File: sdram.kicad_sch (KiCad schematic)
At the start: 25 parts, among them U1 MT48LC16M16A2P, U8 T20Q144xx, X2 ECS-2520MV-250-CM

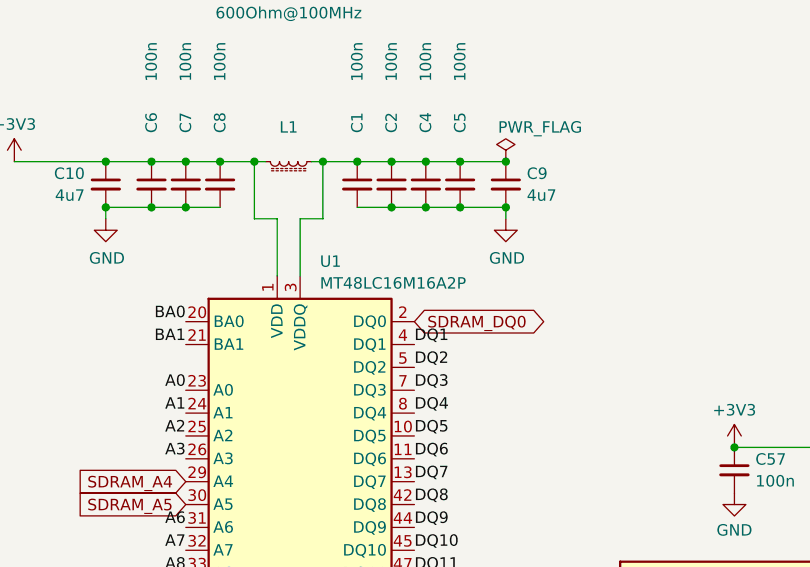
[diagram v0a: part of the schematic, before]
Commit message: part-info update
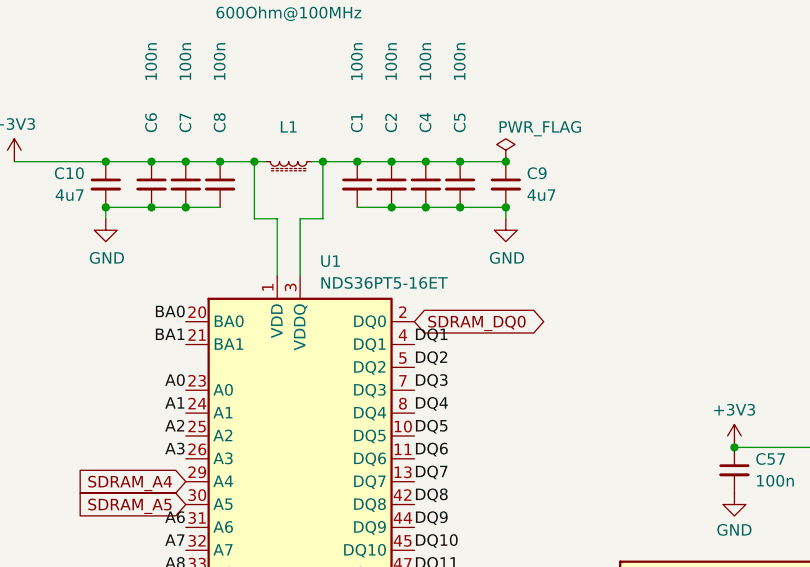
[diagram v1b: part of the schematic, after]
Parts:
- U1: value MT48LC16M16A2P -> NDS36PT5-16ET
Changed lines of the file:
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@@
       (effects (font (size 1.27 1.27)) (justify left))
     )
-    (property "Value" "MT48LC16M16A2P" (at 59.3441 54.1599 0)
+    (property "Value" "NDS36PT5-16ET" (at 59.3441 54.1599 0)
       (effects (font (size 1.27 1.27)) (justify left))
     )
@@
       (effects (font (size 1.27 1.27) italic) hide)
     )
-    (property "Datasheet" "https://www.micron.com/-/media/client/global/documents/products/data-sheet/dram/256mb_sdr.pdf" (at 57.15 95.25 0)
+    (property "Datasheet" "" (at 57.15 95.25 0)
       (effects (font (size 1.27 1.27)) hide)
     )

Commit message: Added Manufacturer + Part info for most components.
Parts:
- C1, C12, C13, C15, C2, C3, C4, C42, C5, C57, C6, C64, C7, C8: Manufacturer (none) -> Samsung; Part (none) -> CL10B104KB8NFN
- C10, C9: Manufacturer (none) -> TDK; Part (none) -> 2012X5R1C475K125AC
- L1: Manufacturer (none) -> Laird; Part (none) -> MI0603J601R-10
- U1: Manufacturer (none) -> Insignis; Part (none) -> NDS36PT5-16ET
- U8: Manufacturer (none) -> Efinix; Part (none) -> T20Q144C4
- X2: Manufacturer (none) -> ECS; Part (none) -> ECS-2520MV-250-CL-TR
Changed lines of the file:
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@@
+      (effects (font (size 1.27 1.27)) hide)
+    )
+    (property "Manufacturer" "TDK" (at 80.01 43.18 0)
+      (effects (font (size 1.27 1.27)) hide)
+    )
+    (property "Part" "2012X5R1C475K125AC" (at 80.01 43.18 0)
       (effects (font (size 1.27 1.27)) hide)
     )
@@
     )
     (property "Datasheet" "https://www.efinixinc.com/docs/trion8-ds-v4.4.pdf" (at 118.11 119.38 0)
+      (effects (font (size 1.27 1.27)) hide)
+    )
+    (property "Manufacturer" "Efinix" (at 118.11 92.71 0)
+      (effects (font (size 1.27 1.27)) hide)
+    )
+    (property "Part" "T20Q144C4" (at 118.11 92.71 0)
       (effects (font (size 1.27 1.27)) hide)
     )
@@
       (effects (font (size 1.27 1.27)) hide)
     )
+    (property "Manufacturer" "Samsung" (at 74.93 43.18 0)
+      (effects (font (size 1.27 1.27)) hide)
+    )
+    (property "Part" "CL10B104KB8NFN" (at 74.93 43.18 0)
+      (effects (font (size 1.27 1.27)) hide)
+    )
     (pin "1")
     (pin "2")
@@
       (effects (font (size 1.27 1.27)) hide)
     )
+    (property "Manufacturer" "Samsung" (at 48.26 43.18 0)
+      (effects (font (size 1.27 1.27)) hide)
+    )
+    (property "Part" "CL10B104KB8NFN" (at 48.26 43.18 0)
+      (effects (font (size 1.27 1.27)) hide)
+    )
     (pin "1")
     (pin "2")
@@
       (effects (font (size 1.27 1.27)) hide)
     )
+    (property "Manufacturer" "Samsung" (at 265.43 144.78 0)
+      (effects (font (size 1.27 1.27)) hide)
+    )
+    (property "Part" "CL10B104KB8NFN" (at 265.43 144.78 0)
+      (effects (font (size 1.27 1.27)) hide)
+    )
     (pin "1")
     (pin "2")
@@
     )
     (property "Datasheet" "~" (at 265.43 114.3 0)
+      (effects (font (size 1.27 1.27)) hide)
+    )
+    (property "Manufacturer" "Samsung" (at 265.43 114.3 0)
+      (effects (font (size 1.27 1.27)) hide)
+    )
+    (property "Part" "CL10B104KB8NFN" (at 265.43 114.3 0)
       (effects (font (size 1.27 1.27)) hide)
     )
@@
     )
     (property "Datasheet" "~" (at 105.41 74.93 0)
+      (effects (font (size 1.27 1.27)) hide)
+    )
+    (property "Manufacturer" "Samsung" (at 105.41 74.93 0)
+      (effects (font (size 1.27 1.27)) hide)
+    )
+    (property "Part" "CL10B104KB8NFN" (at 105.41 74.93 0)
       (effects (font (size 1.27 1.27)) hide)
     )
@@
       (effects (font (size 1.27 1.27)) hide)
     )
+    (property "Manufacturer" "Laird" (at 55.88 40.64 0)
+      (effects (font (size 1.27 1.27)) hide)
+    )
+    (property "Part" "MI0603J601R-10" (at 55.88 40.64 0)
+      (effects (font (size 1.27 1.27)) hide)
+    )
     (pin "2")
     (pin "1")
@@
     )
     (property "Datasheet" "https://www.efinixinc.com/docs/trion8-ds-v4.4.pdf" (at 187.96 114.3 0)
+      (effects (font (size 1.27 1.27)) hide)
+    )
+    (property "Manufacturer" "Efinix" (at 187.96 87.63 0)
+      (effects (font (size 1.27 1.27)) hide)
+    )
+    (property "Part" "T20Q144C4" (at 187.96 87.63 0)
       (effects (font (size 1.27 1.27)) hide)
     )
@@
       (effects (font (size 1.27 1.27)) hide)
     )
+    (property "Manufacturer" "TDK" (at 35.56 43.18 0)
+      (effects (font (size 1.27 1.27)) hide)
+    )
+    (property "Part" "2012X5R1C475K125AC" (at 35.56 43.18 0)
+      (effects (font (size 1.27 1.27)) hide)
+    )
     (pin "1")
     (pin "2")
@@
     )
     (property "Datasheet" "https://www.efinixinc.com/docs/trion8-ds-v4.4.pdf" (at 80.01 198.12 0)
+      (effects (font (size 1.27 1.27)) hide)
+    )
+    (property "Manufacturer" "Efinix" (at 80.01 171.45 0)
+      (effects (font (size 1.27 1.27)) hide)
+    )
+    (property "Part" "T20Q144C4" (at 80.01 171.45 0)
       (effects (font (size 1.27 1.27)) hide)
     )
@@
       (effects (font (size 1.27 1.27)) hide)
     )
+    (property "Manufacturer" "Samsung" (at 152.4 167.64 0)
+      (effects (font (size 1.27 1.27)) hide)
+    )
+    (property "Part" "CL10B104KB8NFN" (at 152.4 167.64 0)
+      (effects (font (size 1.27 1.27)) hide)
+    )
     (pin "1")
     (pin "2")
@@
     )
     (property "Datasheet" "https://www.efinixinc.com/docs/trion8-ds-v4.4.pdf" (at 189.23 144.78 0)
+      (effects (font (size 1.27 1.27)) hide)
+    )
+    (property "Manufacturer" "Efinix" (at 189.23 118.11 0)
+      (effects (font (size 1.27 1.27)) hide)
+    )
+    (property "Part" "T20Q144C4" (at 189.23 118.11 0)
       (effects (font (size 1.27 1.27)) hide)
     )
@@
       (effects (font (size 1.27 1.27)) hide)
     )
+    (property "Manufacturer" "Samsung" (at 40.64 43.18 0)
+      (effects (font (size 1.27 1.27)) hide)
+    )
+    (property "Part" "CL10B104KB8NFN" (at 40.64 43.18 0)
+      (effects (font (size 1.27 1.27)) hide)
+    )
     (pin "1")
     (pin "2")
@@
     )
     (property "Datasheet" "" (at 57.15 95.25 0)
+      (effects (font (size 1.27 1.27)) hide)
+    )
+    (property "Manufacturer" "Insignis" (at 57.15 88.9 0)
+      (effects (font (size 1.27 1.27)) hide)
+    )
+    (property "Part" "NDS36PT5-16ET" (at 57.15 88.9 0)
       (effects (font (size 1.27 1.27)) hide)
     )
@@
       (effects (font (size 1.27 1.27)) hide)
     )
+    (property "Manufacturer" "Samsung" (at 264.16 81.28 0)
+      (effects (font (size 1.27 1.27)) hide)
+    )
+    (property "Part" "CL10B104KB8NFN" (at 264.16 81.28 0)
+      (effects (font (size 1.27 1.27)) hide)
+    )
     (pin "1")
     (pin "2")
@@
     )
     (property "Datasheet" "https://www.efinixinc.com/docs/trion8-ds-v4.4.pdf" (at 187.96 81.28 0)
+      (effects (font (size 1.27 1.27)) hide)
+    )
+    (property "Manufacturer" "Efinix" (at 187.96 54.61 0)
+      (effects (font (size 1.27 1.27)) hide)
+    )
+    (property "Part" "T20Q144C4" (at 187.96 54.61 0)
       (effects (font (size 1.27 1.27)) hide)
     )
@@
       (effects (font (size 1.27 1.27)) hide)
     )
+    (property "Manufacturer" "Efinix" (at 187.96 151.13 0)
+      (effects (font (size 1.27 1.27)) hide)
+    )
+    (property "Part" "T20Q144C4" (at 187.96 151.13 0)
+      (effects (font (size 1.27 1.27)) hide)
+    )
     (pin "76")
     (pin "141")
@@
       (effects (font (size 1.27 1.27)) hide)
     )
+    (property "Manufacturer" "ECS" (at 138.43 168.91 0)
+      (effects (font (size 1.27 1.27)) hide)
+    )
+    (property "Part" "ECS-2520MV-250-CL-TR" (at 138.43 168.91 0)
+      (effects (font (size 1.27 1.27)) hide)
+    )
     (pin "1")
     (pin "2")
@@
       (effects (font (size 1.27 1.27)) hide)
     )
+    (property "Manufacturer" "Samsung" (at 44.45 43.18 0)
+      (effects (font (size 1.27 1.27)) hide)
+    )
+    (property "Part" "CL10B104KB8NFN" (at 44.45 43.18 0)
+      (effects (font (size 1.27 1.27)) hide)
+    )
     (pin "1")
     (pin "2")
@@
     )
     (property "Datasheet" "~" (at 264.16 33.02 0)
+      (effects (font (size 1.27 1.27)) hide)
+    )
+    (property "Manufacturer" "Samsung" (at 264.16 33.02 0)
+      (effects (font (size 1.27 1.27)) hide)
+    )
+    (property "Part" "CL10B104KB8NFN" (at 264.16 33.02 0)
       (effects (font (size 1.27 1.27)) hide)
     )
@@
       (effects (font (size 1.27 1.27)) hide)
     )
+    (property "Manufacturer" "Samsung" (at 71.12 43.18 0)
+      (effects (font (size 1.27 1.27)) hide)
+    )
+    (property "Part" "CL10B104KB8NFN" (at 71.12 43.18 0)
+      (effects (font (size 1.27 1.27)) hide)
+    )
     (pin "1")
     (pin "2")
@@
       (effects (font (size 1.27 1.27)) hide)
     )
+    (property "Manufacturer" "Samsung" (at 67.31 43.18 0)
+      (effects (font (size 1.27 1.27)) hide)
+    )
+    (property "Part" "CL10B104KB8NFN" (at 67.31 43.18 0)
+      (effects (font (size 1.27 1.27)) hide)
+    )
     (pin "1")
     (pin "2")
@@
     )
     (property "Datasheet" "~" (at 62.23 153.67 0)
+      (effects (font (size 1.27 1.27)) hide)
+    )
+    (property "Manufacturer" "Samsung" (at 62.23 153.67 0)
+      (effects (font (size 1.27 1.27)) hide)
+    )
+    (property "Part" "CL10B104KB8NFN" (at 62.23 153.67 0)
       (effects (font (size 1.27 1.27)) hide)
     )
@@
       (effects (font (size 1.27 1.27)) hide)
     )
+    (property "Manufacturer" "Samsung" (at 63.5 43.18 0)
+      (effects (font (size 1.27 1.27)) hide)
+    )
+    (property "Part" "CL10B104KB8NFN" (at 63.5 43.18 0)
+      (effects (font (size 1.27 1.27)) hide)
+    )

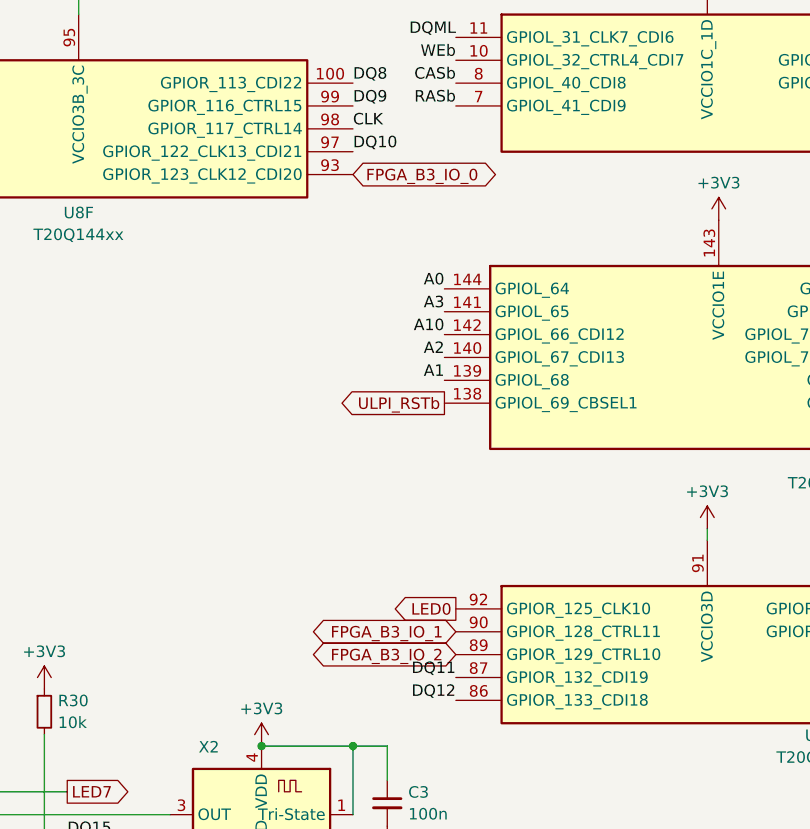
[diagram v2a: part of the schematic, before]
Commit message: Added GPS receiver; increased board size
including battery supply; made board bigger
and added edge connectors for ETH GPIO, PPS
and antenna.
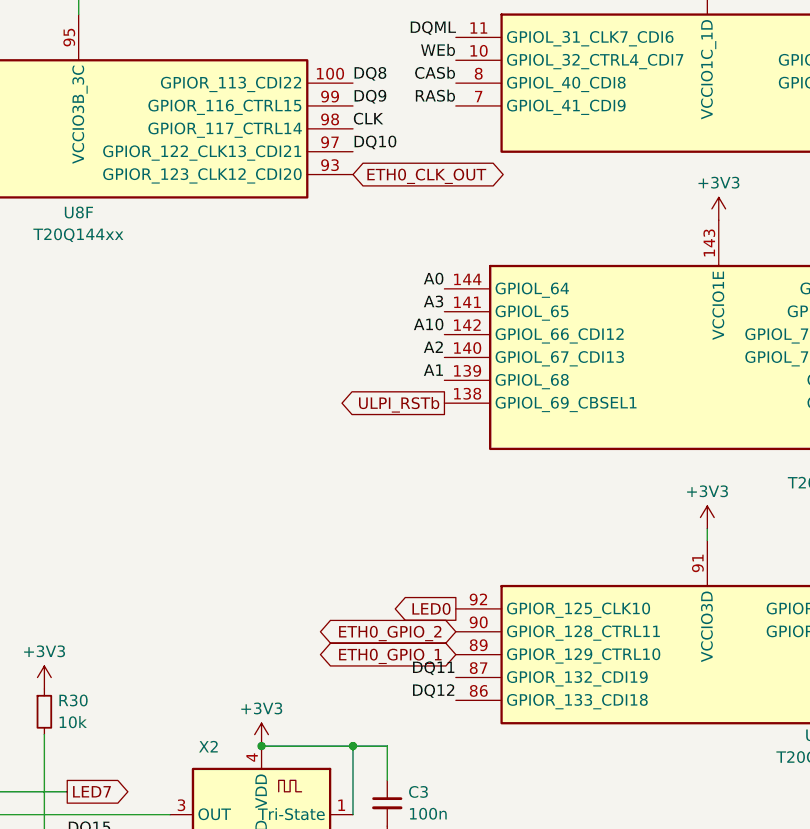
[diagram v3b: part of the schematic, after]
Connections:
- net FPGA_B3_IO_0 renamed ETH0_CLK_OUT
- net FPGA_B3_IO_1 renamed ETH0_GPIO_2
- net FPGA_B3_IO_2 renamed ETH0_GPIO_1
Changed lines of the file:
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@@
     )
   )
-  (global_label "FPGA_B3_IO_0" (shape bidirectional) (at 148.59 97.79 0) (fields_autoplaced)
+  (global_label "ETH0_GPIO_2" (shape bidirectional) (at 160.02 148.59 180) (fields_autoplaced)
+    (effects (font (size 1.27 1.27)) (justify right))
+    (property "Intersheetrefs" "${INTERSHEET_REFS}" (at 143.6469 148.59 0)
+      (effects (font (size 1.27 1.27)) (justify right) hide)
+    )
+  )
+  (global_label "ETH0_CLK_OUT" (shape bidirectional) (at 148.59 97.79 0) (fields_autoplaced)
     (effects (font (size 1.27 1.27)) (justify left))
-    (property "Intersheetrefs" "${INTERSHEET_REFS}" (at 165.9308 97.79 0)
+    (property "Intersheetrefs" "${INTERSHEET_REFS}" (at 166.475 97.79 0)
       (effects (font (size 1.27 1.27)) (justify left) hide)
     )
@@
     )
   )
-  (global_label "FPGA_B3_IO_1" (shape bidirectional) (at 160.02 148.59 180) (fields_autoplaced)
-    (effects (font (size 1.27 1.27)) (justify right))
-    (property "Intersheetrefs" "${INTERSHEET_REFS}" (at 142.6792 148.59 0)
-      (effects (font (size 1.27 1.27)) (justify right) hide)
-    )
-  )
-  (global_label "FPGA_B3_IO_2" (shape bidirectional) (at 160.02 151.13 180) (fields_autoplaced)
-    (effects (font (size 1.27 1.27)) (justify right))
-    (property "Intersheetrefs" "${INTERSHEET_REFS}" (at 142.6792 151.13 0)
-      (effects (font (size 1.27 1.27)) (justify right) hide)
-    )
-  )
   (global_label "A12" (shape input) (at 44.45 96.52 180) (fields_autoplaced)
     (effects (font (size 1.27 1.27)) (justify right))
@@
       (effects (font (size 1.27 1.27)) (justify right) hide)
     )
+  )
+  (global_label "ETH0_GPIO_1" (shape bidirectional) (at 160.02 151.13 180) (fields_autoplaced)
+    (effects (font (size 1.27 1.27)) (justify right))
+    (property "Intersheetrefs" "${INTERSHEET_REFS}" (at 143.6469 151.13 0)
+      (effects (font (size 1.27 1.27)) (justify right) hide)
+    )
